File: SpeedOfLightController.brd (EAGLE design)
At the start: 99.7 x 100 mm, 140 parts, among them IC10 74LS595D, IC11 74LS595D, Q10 FDN360P, Q12 FDN360P, Q14 FDN360P, Q16 FDN360P, Q18 FDN360P, Q20 FDN360P, Q22 FDN360P, Q24 FDN360P, Q26 FDN360P, SW2 MOMENTARYBUTTON, U1 ATMEGA328PBTQFP-32, U2 LM380NDIP14, U3 AD5111ADLFCSP10, X1 JST-XH-08-PIN-LONG-PAD, X10 JST-XH-06-PIN-LONG-PAD, X11 JST-XH-06-PIN-LONG-PAD, X12 JST-XH-06-PIN-LONG-PAD, X13 JST-XH-06-PIN-LONG-PAD, X14 JST-XH-07-PIN-LONG-PAD, X15 JST-XH-02-PIN-LONG-PAD, X16 JST-XH-02-PIN-LONG-PAD, X17 JST-XH-02-PIN-LONG-PAD, X18 JST-XH-02-PIN-LONG-PAD, X19 JST-XH-03-PIN-LONG-PAD, X2 JST-XH-08-PIN-LONG-PAD, X20 JST-XH-03-PIN-LONG-PAD, X21 JST-XH-03-PIN-LONG-PAD, X22 JST-XH-03-PIN-LONG-PAD, X3 JST-XH-08-PIN-LONG-PAD, X4 JST-XH-08-PIN-LONG-PAD, X5 JST-XH-08-PIN-LONG-PAD, X6 JST-XH-08-PIN-LONG-PAD, X7 JST-XH-08-PIN-LONG-PAD, X8 JST-XH-08-PIN-LONG-PAD, X9 JST-XH-08-PIN-LONG-PAD

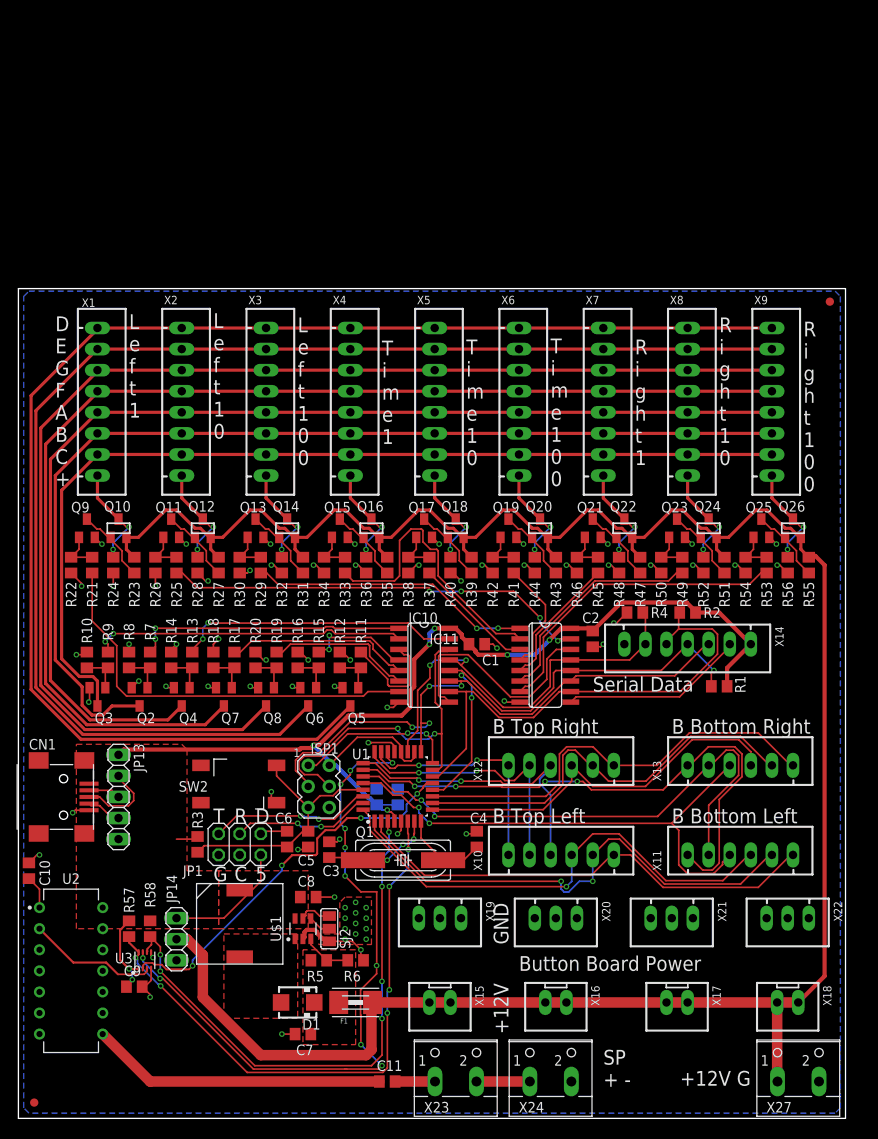
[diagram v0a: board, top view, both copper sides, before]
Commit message: USBPD design review
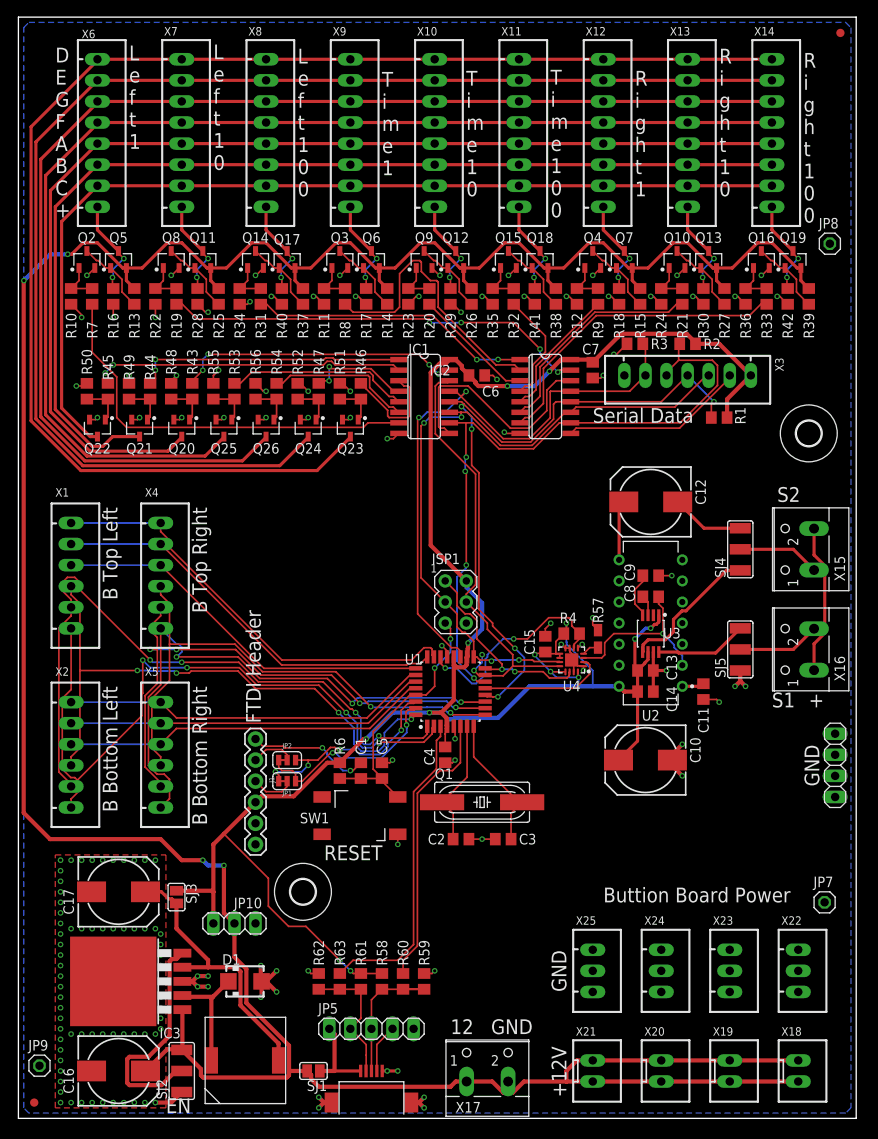
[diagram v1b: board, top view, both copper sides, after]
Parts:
- removed CN1: (no value), adafruit:USB-MINIB
- removed F3: FIDUCIAL, ECE388:FIDUCIAL_1MM
- removed IC10, IC11: 74LS595D, 74xx-us:SO16
- removed JP13: (no value), pinhead:1X05
- removed JP14: (no value), pinhead:1X03
- removed R5: 82K, rcl:R0805
- removed SW2: MOMENTARYBUTTON, ECE388:SPST_NO_SMD
- removed X27: (no value), ECE388:W237-102
- added C14, C15: 0.1uF, rcl:C0805
- added C16: 680uF, rcl:140CLH-0810
- added C17: 220uF, rcl:140CLH-0810
- added H1, H2: MOUNT-HOLE3.0, holes:3,0
- added IC1, IC2: 74LS595D, 74xx-us:SO16
- added IC3: (no value), linear:TO263-5
- added J1: 6_PIN_SERIAL_CABLEPTH, SparkFun-Connectors:FTDI_BASIC
- added JP10: (no value), pinhead:1X03
- added JP2: JUMPER-SMT_3_1-NC_TRACE_SILK, SparkFun-Jumpers:SMT-JUMPER_3_1-NC_TRACE_SILK
- added JP5: (no value), pinhead:1X05
- added JP6: (no value), pinhead:1X04
- added JP7, JP8, JP9: (no value), pinhead:1X01
- added R59, R62: 1K5, rcl:R0805
- added R60, R63: 470, rcl:R0805
- added R61: 10K, rcl:R0805
- added SJ1, SJ3: (no value), ECE388:SJ
- added SJ4, SJ5: (no value), jumper:SJ_2W
- added SW1: MOMENTARYBUTTON, ECE388:SPST_NO_SMD
- added U4: AD5141ADLFCSP3, tmc:QFN50P300X300X80-17T160N
- added X25: JST-XH-03-PIN-LONG-PAD, Rembrandt Electronics - JST XH Connectors v1-0:JST-XH-03-PACKAGE-LONG-PAD
- C1, C4: value (none) -> 0.1uF
- C10, C12: value (none) -> 470uF; device rcl:C0805 -> rcl:140CLH-0810
- C11: value (none) -> 47uF
- C13: value (none) -> 4.7uF
- C2, C3: value (none) -> 22pF
- C7: value 22uF -> 0.1uF
- C8: value 22uF -> 47nF
- C9: value (none) -> 47nF
- F1: value (none) -> FIDUCIAL; device adafruit:1812 -> ECE388:FIDUCIAL_1MM
- JP1: value (none) -> JUMPER-SMT_3_1-NC_TRACE_SILK; device pinhead:2X03 -> SparkFun-Jumpers:SMT-JUMPER_3_1-NC_TRACE_SILK
- Q1: value (none) -> 16MHz
- Q10, Q14, Q16, Q20, Q22, Q24, Q26: value FDN360P -> AO3414SOT23; device transistor-power:SUPER-SOT3 -> tmc:SOT95P240X110-3N
- Q11, Q13, Q17, Q19, Q5, Q6, Q7: value (none) -> AO3415; device adafruit:SOT23 -> tmc:SOT95P240X110-3N
- Q12, Q18: value FDN360P -> AO3415; device transistor-power:SUPER-SOT3 -> tmc:SOT95P240X110-3N
- Q15, Q2, Q21, Q23, Q25, Q3, Q4, Q8, Q9: value (none) -> AO3414SOT23; device adafruit:SOT23 -> tmc:SOT95P240X110-3N
- R11, R17, R23, R29, R35, R41, R49, R51, R55: value 1K -> 10K
- R14, R20, R26, R32, R38, R44, R46, R54, R8: value 10K -> 1K
- R57: value 10K -> 0; device rcl:R0805 -> rcl:R0805W
- R6: value 4.3K -> 10K
- SJ2: device jumper:SJ_2 -> jumper:SJ_2W
- U$1: value MT3608SOT23-6 -> USBMICRO; device tmc:SOT95P280X110-6N -> tmc:USBMICRO
- U3: value AD5111ADLFCSP10 -> SSM2305ADMSOP8_2; device tmc:SON50P200X200X80-9T100X160N -> tmc:SOP65P490X95-8N
- X1, X2, X4, X5: value JST-XH-08-PIN-LONG-PAD -> JST-XH-06-PIN-LONG-PAD; device Rembrandt Electronics - JST XH Connectors v1-0:JST-XH-08-PACKAGE-LONG-PAD -> Rembrandt Electronics - JST XH Connectors v1-0:JST-XH-06-PACKAGE-LONG-PAD
- X10, X11, X12, X13: value JST-XH-06-PIN-LONG-PAD -> JST-XH-08-PIN-LONG-PAD; device Rembrandt Electronics - JST XH Connectors v1-0:JST-XH-06-PACKAGE-LONG-PAD -> Rembrandt Electronics - JST XH Connectors v1-0:JST-XH-08-PACKAGE-LONG-PAD
- X14: value JST-XH-07-PIN-LONG-PAD -> JST-XH-08-PIN-LONG-PAD; device Rembrandt Electronics - JST XH Connectors v1-0:JST-XH-07-PACKAGE-LONG-PAD -> Rembrandt Electronics - JST XH Connectors v1-0:JST-XH-08-PACKAGE-LONG-PAD
- X15, X16, X17: value JST-XH-02-PIN-LONG-PAD -> (none); device Rembrandt Electronics - JST XH Connectors v1-0:JST-XH-02-PACKAGE-LONG-PAD -> ECE388:W237-102
- X19, X20, X21: value JST-XH-03-PIN-LONG-PAD -> JST-XH-02-PIN-LONG-PAD; device Rembrandt Electronics - JST XH Connectors v1-0:JST-XH-03-PACKAGE-LONG-PAD -> Rembrandt Electronics - JST XH Connectors v1-0:JST-XH-02-PACKAGE-LONG-PAD
- X23, X24: value (none) -> JST-XH-03-PIN-LONG-PAD; device ECE388:W237-102 -> Rembrandt Electronics - JST XH Connectors v1-0:JST-XH-03-PACKAGE-LONG-PAD
- X3: value JST-XH-08-PIN-LONG-PAD -> JST-XH-07-PIN-LONG-PAD; device Rembrandt Electronics - JST XH Connectors v1-0:JST-XH-08-PACKAGE-LONG-PAD -> Rembrandt Electronics - JST XH Connectors v1-0:JST-XH-07-PACKAGE-LONG-PAD
- moved F1 130.6 mm to (99.1, 130.8)
- moved X11 91.0 mm to (60.3, 118.7), turned to 270 degrees
- moved X10 88.3 mm to (50.2, 118.7), turned to 270 degrees
- moved C7 87.3 mm to (69.2, 90.2), turned to 270 degrees
- moved U2 81.5 mm to (76.2, 59.7), turned to 180 degrees
- moved R3 80.1 mm to (74.3, 93.3), turned to 0 degrees
- moved C9 79.5 mm to (76.2, 65.4), turned to 180 degrees
- moved R21 78.1 mm to (80.0, 99.1)
- moved X13 76.5 mm to (80.6, 118.7), turned to 270 degrees
- moved X12 76.4 mm to (70.5, 118.7), turned to 270 degrees
- moved C10 75.5 mm to (75.6, 43.2), turned to 180 degrees
- moved R55 74.8 mm to (23.5, 87.6), turned to 270 degrees
- moved Q10 74.7 mm to (79.4, 103.5), turned to 90 degrees
- moved R24 73.6 mm to (77.5, 99.1)
- moved R9 73.5 mm to (69.8, 99.1), turned to 90 degrees
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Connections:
- removed net N$26: C11.2, X23.1
- removed net N$33: C7.1, D1.C, F1.1, R5.2
- removed net SOUND_C: R58.1, U1.3, U3.6
- removed net SOUND_UD: U1.22, U3.7
- new net ADSOUND+: SJ4.1, U3.5
- new net ADSOUND-: SJ5.3, U3.8
- new net D+: JP5.3, R58.1, R59.2, R60.2, U$1.P$3
- new net D-: JP5.2, R61.2, R62.1, R63.1, U$1.P$2
- new net FTDIRX: J1.TXO, JP1.2
- new net FTDITX: J1.RXI, JP2.2
- new net LMSOUND: C12.-, SJ4.3
- new net N$40: IC3.5, SJ2.2
- new net N$41: C17.+, IC3.4, L1.P$2, SJ3.2
- new net SOUND+: SJ4.2, X15.1
- new net SOUND-: SJ5.2, X16.2
- new net UCD+: R60.1, U1.6
- new net UCD-: R63.2, U1.3
- net +12V: now also C16.+, IC3.1, JP10.2, Q11.2, Q13.2, Q17.2, Q19.2, Q5.2, Q6.2, Q7.2, R13.2, R14.2, R15.2, R25.2, R26.2, R37.2, R38.2, SJ1.2, SJ2.3, X19.1, X19.2, X20.1, X20.2, X21.1, X21.2; no longer F1.2, JP14.2, Q10.2, Q14.2, Q16.2, Q20.2, Q22.2, Q24.2, Q26.2, R23.2, R31.2, R35.2, R43.2, R47.2, R51.2, R55.2, X15.1, X15.2, X16.1, X16.2, X17.2, X27.1
- net +5V: now also C10.+, C14.2, C15.1, C4.2, C6.1, C7.1, IC1.16, IC2.16, J1.VCC, JP10.1, R4.2, R6.2, R61.1, SJ3.1, U3.6, U4.10, U4.13, U4.16, U4.9, X3.1; no longer C1.1, C12.2, C2.1, C8.1, C9.1, CN1.VBUS, IC10.16, IC11.16, JP1.5, JP13.1, JP14.1, L1.P$1, R3.2, R57.2, SJ2.3, U$1.5, X14.1
- net A: now also Q20.3, X10.5, X11.5, X12.5, X13.5, X14.5; no longer Q4.3, X1.5, X2.5, X3.5, X4.5, X5.5
- net AN1: now also IC1.7, R7.1; no longer IC10.7, R21.1
- net AN2: now also IC2.15, R19.1; no longer IC11.15, R25.1
- net AN3: now also IC2.1, R31.1; no longer IC11.1, R29.1
- net AN4: now also IC2.2, R8.1; no longer IC11.2, R33.1
- net AN5: now also IC2.3, R20.1; no longer IC11.3, R37.1
- net AN6: now also IC2.4, R32.1; no longer IC11.4, R41.1
- net AN7: now also IC2.5, R9.1; no longer IC11.5, R45.1
- net AN8: now also IC2.6, R21.1; no longer IC11.6, R49.1
- net AN9: now also IC2.7, R33.1; no longer IC11.7, R53.1
- net B: now also Q21.3, X10.6, X11.6, X12.6, X13.6, X14.6; no longer Q2.3, X1.6, X2.6, X3.6, X4.6, X5.6
- net B_COL_0: now also X1.4, X2.4; no longer X10.4, X11.4
- net B_COL_1: now also X1.5, X2.5; no longer X10.5, X11.5
- net B_COL_2: now also X1.6, X2.6; no longer X10.6, X11.6
- net B_COL_3: now also X4.4, X5.4; no longer X12.4, X13.4
- net B_COL_4: now also X4.5, X5.5; no longer X12.5, X13.5
- net B_COL_5: now also X4.6, X5.6; no longer X12.6, X13.6
- net B_ROW_0: now also X1.1, X4.1; no longer X10.1, X12.1
- net B_ROW_1: now also X1.2, X4.2; no longer X10.2, X12.2
- net B_ROW_2: now also X1.3, X4.3; no longer X10.3, X12.3
- net B_ROW_3: now also X2.1, X5.1; no longer X11.1, X13.1
- net B_ROW_4: now also X2.2, X5.2; no longer X11.2, X13.2
- net B_ROW_5: now also X2.3, X5.3; no longer X11.3, X13.3
- net C: now also Q22.3, X10.7, X11.7, X12.7, X13.7, X14.7; no longer Q3.3, X1.7, X2.7, X3.7, X4.7, X5.7
- net D: now also Q23.3, X10.1, X11.1, X12.1, X13.1, X14.1; no longer Q5.3, X1.1, X2.1, X3.1, X4.1, X5.1
- net DTR: now also C1.2, J1.DTR; no longer C6.2, JP1.6
- net E: now also Q24.3, X10.2, X11.2, X12.2, X13.2, X14.2; no longer Q6.3, X1.2, X2.2, X3.2, X4.2, X5.2
- net F: now also Q25.3, X10.4, X11.4, X12.4, X13.4, X14.4; no longer Q7.3, X1.4, X2.4, X3.4, X4.4, X5.4
- net G: now also Q26.3, X10.3, X11.3, X12.3, X13.3, X14.3; no longer Q8.3, X1.3, X2.3, X3.3, X4.3, X5.3
- net GND: now also C10.-, C11.2, C14.1, C15.2, C16.-, C17.-, C2.1, C6.2, C9.1, D1.A, IC1.8, IC2.8, IC3.3, IC3.6, J1.CTS, J1.GND, JP10.3, JP5.5, JP6.1, JP6.2, JP6.3, JP6.4, JP7.1, JP8.1, JP9.1, Q10.2, Q14.2, Q16.2, Q20.2, Q22.2, Q24.2, Q26.2, R11.1, R17.1, R23.1, R29.1, R3.1, R35.1, R41.1, R49.1, R51.1, R55.1, R57.1, R59.1, R62.2, SJ5.1, SW1.1, U$1.P$5, U$1.P$6, U$1.P$8, U3.7, U4.1, U4.15, U4.17, U4.5, U4.7, U4.8, X17.2, X23.1, X23.2, X23.3, X24.1, X24.3, X25.1, X25.2, X25.3, X3.7; no longer C1.2, C10.2, C12.1, C2.2, C8.2, C9.2, CN1.GND, IC10.8, IC11.8, JP1.1, JP1.3, JP13.5, JP14.3, Q11.2, Q13.2, Q17.2, Q19.2, Q5.2, Q6.2, Q7.2, R14.1, R20.1, R26.1, R32.1, R38.1, R4.1, R44.1, R46.1, R54.1, R6.1, R8.1, SW2.1, U$1.2, U3.4, U3.5, X14.7, X19.1, X19.2, X19.3, X20.1, X20.2, X20.3, X21.1, X21.2, X21.3, X27.2
- net LED_B: now also IC1.10, IC2.10, X3.5; no longer IC10.10, IC11.10, X14.5
- net LED_D_OUT: now also IC2.9, X3.2; no longer IC11.9, X14.2
- net LED_L: now also IC1.12, IC2.12, X3.4; no longer IC10.12, IC11.12, X14.4
- net LED_O: now also IC1.13, IC2.13, R3.2, X3.6; no longer IC10.13, IC11.13, R4.2, X14.6
- net MISO: now also U4.14
- net MOSI: now also IC1.14, U4.12; no longer IC10.14
- net N$1: now also Q21.1, R44.2, R49.2; no longer Q2.1, R7.2, R8.2
- net N$10: now also Q14.1, R31.2, R34.2; no longer Q13.1, R29.2, R30.2
- net N$11: now also Q3.1, R11.2, R8.2; no longer Q15.1, R33.2, R34.2
- net N$12: now also Q9.1, R20.2, R23.2; no longer Q17.1, R37.2, R38.2
- net N$13: now also Q15.1, R32.2, R35.2; no longer Q19.1, R41.2, R42.2
- net N$14: now also Q4.1, R12.2, R9.2; no longer Q21.1, R45.2, R46.2
- net N$15: now also Q10.1, R21.2, R24.2; no longer Q23.1, R49.2, R50.2
- net N$16: now also Q16.1, R33.2, R36.2; no longer Q25.1, R53.2, R54.2
- net N$17: now also C2.2; no longer C3.2
- net N$18: now also C3.2; no longer C4.2
- net N$19: now also JP5.1, SJ1.1, U$1.P$1; no longer R5.1, R6.2, U$1.3
- net N$2: now also Q22.1, R45.2, R50.2; no longer Q3.1, R10.2, R9.2
- net N$20: now also X15.2, X16.1; no longer X23.2, X24.1
- net N$21: now also C12.+, U2.8; no longer CN1.D+, JP13.2
- net N$22: now also C11.1; no longer C10.1
- net N$23: now also C9.2, U3.4; no longer CN1.D-, JP13.3
- net N$24: now also C8.2, U3.3; no longer D1.A, L1.P$2, U$1.1
- net N$25: now also R57.2, U4.4; no longer C11.1, U2.8
- net N$27: now also Q16.3, Q19.1, R39.1; no longer Q25.3, Q26.1, R55.1
- net N$28: now also Q10.3, Q13.1, R27.1; no longer Q23.3, Q24.1, R51.1
- net N$29: now also Q4.3, Q7.1, R15.1; no longer Q21.3, Q22.1, R47.1
- net N$3: now also Q23.1, R46.2, R51.2; no longer Q5.1, R11.2, R12.2
- net N$30: now also Q3.3, Q6.1, R14.1; no longer Q15.3, Q16.1, R35.1
- net N$31: now also JP5.4, U$1.P$4; no longer CN1.ID, JP13.4
- net N$32: now also D1.C, IC3.2, L1.P$1; no longer SJ2.2, U$1.4
- net N$34: now also Q12.1, Q9.3, R26.1; no longer Q17.3, Q18.1, R39.1
- net N$35: now also Q15.3, Q18.1, R38.1; no longer Q19.3, Q20.1, R43.1
- net N$36: now also Q14.3, Q17.1, R37.1; no longer Q13.3, Q14.1, R31.1
- net N$37: now also Q11.1, Q8.3, R25.1; no longer Q11.3, Q12.1, R27.1
- net N$38: now also Q2.3, Q5.1, R13.1; no longer Q10.1, Q9.3, R23.1
- net N$39: now also IC1.9, IC2.14; no longer IC10.9, IC11.14
- net N$4: now also Q24.1, R47.2, R52.2; no longer Q6.1, R15.2, R16.2
- net N$5: now also Q20.1, R43.2, R48.2; no longer Q4.1, R13.2, R14.2
- net N$6: now also Q25.1, R53.2, R55.2; no longer Q7.1, R17.2, R18.2
- net N$7: now also Q26.1, R54.2, R56.2; no longer Q8.1, R19.2, R20.2
- net N$8: now also Q2.1, R10.2, R7.2; no longer Q9.1, R21.2, R22.2
- net N$9: now also Q8.1, R19.2, R22.2; no longer Q11.1, R25.2, R26.2
- net RX: now also JP1.3, JP2.1; no longer JP1.2
- net SCK: now also IC1.11, IC2.11, U4.11, X3.3; no longer IC10.11, IC11.11, X14.3
- net SCORE0_1: now also Q5.3, R16.2, X6.8; no longer Q10.3, R24.2, X1.8
- net SCORE0_10: now also Q11.3, X7.8; no longer Q12.3, X2.8
- net SCORE0_100: now also Q17.3, R40.2, X8.8; no longer Q14.3, R32.2, X3.8
- net SCORE1_1: now also Q6.3, R17.2, X9.8; no longer Q16.3, R36.2, X4.8
- net SCORE1_10: now also Q12.3, R29.2, X10.8; no longer Q18.3, R40.2, X5.8
- net SCORE1_100: now also Q18.3, R41.2, X11.8; no longer Q20.3, R44.2, X6.8
- net SCORE2_1: now also Q7.3, R18.2, X12.8; no longer Q22.3, R48.2, X7.8
- net SCORE2_10: now also Q13.3, R30.2, X13.8; no longer Q24.3, R52.2, X8.8
- net SCORE2_100: now also Q19.3, R42.2, X14.8; no longer Q26.3, R56.2, X9.8
- net SIGA: now also IC1.15, R43.1; no longer IC10.15, R13.1
- net SIGB: now also IC1.1, R44.1; no longer IC10.1, R7.1
- net SIGC: now also IC1.2, R45.1; no longer IC10.2, R9.1
- net SIGD: now also IC1.3, R46.1; no longer IC10.3, R11.1
- net SIGE: now also IC1.4, R47.1; no longer IC10.4, R15.1
- net SIGF: now also IC1.5, R53.1; no longer IC10.5, R17.1
- net SIGG: now also IC1.6, R54.1; no longer IC10.6, R19.1
- net SOUNDOUT: now also U4.2; no longer U3.2
- net SOUND_ATND: now also C8.1, U4.3; no longer U3.3
- net SOUND_CS: now also R4.1, U1.22, U4.6; no longer R57.1, U1.6, U3.8
- net TX: now also JP1.1, JP2.3; no longer JP1.4
- net UC_RESET: now also C1.1, R6.1, SW1.3; no longer C6.1, R3.1, SW2.3
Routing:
- net +12V: track 283.9 -> 381.0 mm, vias 0 -> 4
- net +5V: track 166.4 -> 261.0 mm, vias 8 -> 13
- net SOUND_UD: track 83.4 -> 0.00 mm, vias 11 -> 0
- net SOUND_C: track 67.2 -> 0.00 mm, vias 6 -> 0
- net SOUND_CS: track 70.6 -> 26.2 mm, vias 6 -> 2
- net UCD-: track 0.00 -> 38.0 mm
- net N$25: track 35.7 -> 2.05 mm
- net UCD+: track 0.00 -> 33.5 mm
- net N$41: track 0.00 -> 33.4 mm
- net GND: track 102.5 -> 135.3 mm, vias 71 -> 148
- net SOUNDOUT: track 47.4 -> 15.3 mm, vias 4 -> 0
- net N$40: track 0.00 -> 27.5 mm
- net B_COL_2: track 57.4 -> 83.6 mm, vias 0 -> 4
- net B_ROW_0: track 28.2 -> 53.2 mm, vias 2 -> 0
- net B_ROW_3: track 69.0 -> 44.5 mm, vias 4 -> 0
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- removed copper zone on layer 1, net +5V
- removed copper zone on layer 1, net N$24
- removed copper zone on layer 1, net N$33
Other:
- board size 99.7 x 100 mm -> 101 x 132.7 mm
- board text added: "+"
- board text added: "12 GND"
- board text added: "Buttion Board Power"
- board text added: "EN"
- board text added: "FTDI Header"
- board text added: "RESET"
- board text added: "S1"
- board text added: "S2"
- board text removed: "+12V G"
- board text removed: "5"
- board text removed: "Button Board Power"
- board text removed: "C"
- board text removed: "D"
- board text removed: "G"
- board text removed: "R"
- board text removed: "SP + -"
- board text removed: "T"
